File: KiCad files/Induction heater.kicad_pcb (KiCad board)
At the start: 2 copper layers, 100 x 100 mm, 31 parts, among them J1 PWR_IN, Q1 NMOS, Q2 NMOS, Q3 2N7000, Q4 2N7000, Q5 2N7000

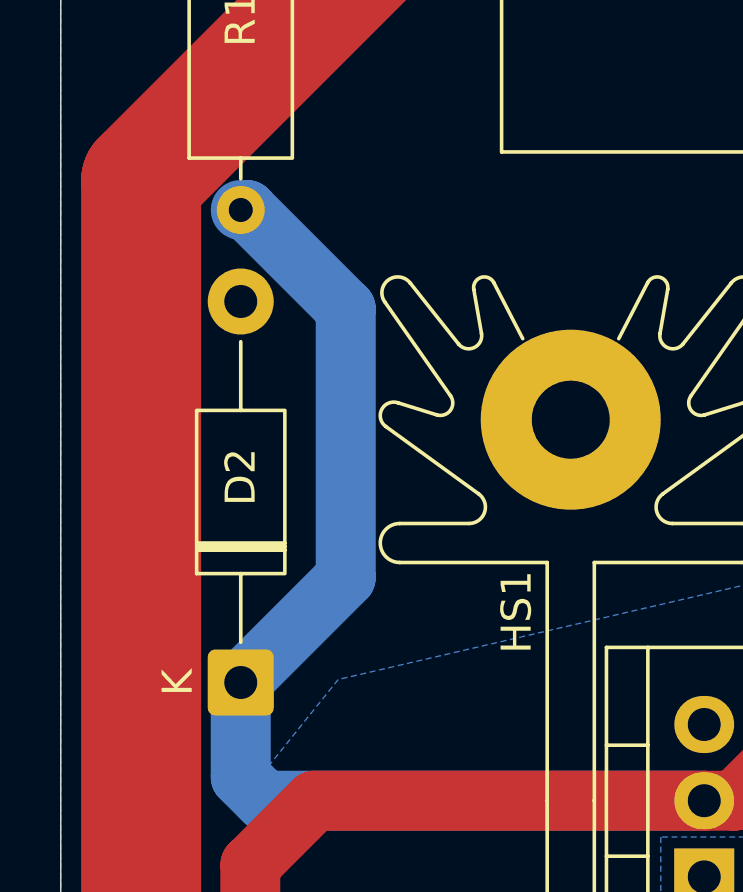
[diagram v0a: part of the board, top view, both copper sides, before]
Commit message: Update
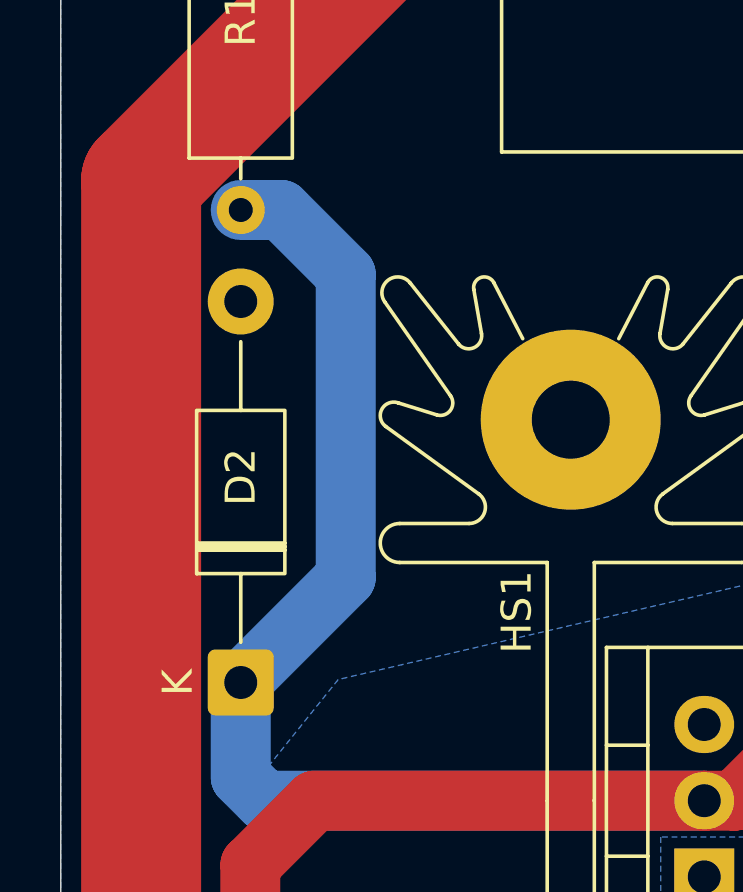
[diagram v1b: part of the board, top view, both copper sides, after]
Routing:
- net G2: track 148.5 -> 191.5 mm
- net G1: track 111.4 -> 150.4 mm
- net Net-(D3-K): track 68.3 -> 95.8 mm
- net Net-(D1-K): track 65.9 -> 78.0 mm
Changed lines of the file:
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@@
+	)
+	(segment
+		(start 104.22875 76.07625)
+		(end 110.555 69.75)
+		(width 3)
+		(layers "B.Cu" "B.Mask")
+		(solder_mask_margin 0)
+		(net 1)
 	)
 	(segment
@@
 	)
 	(segment
+		(start 101 76)
+		(end 104.1525 76)
+		(width 3)
+		(layers "B.Cu" "B.Mask")
+		(solder_mask_margin 0)
+		(net 1)
+	)
+	(segment
 		(start 108.25 118.35)
 		(end 107.35 119.25)
@@
 	)
 	(segment
+		(start 64.291315 76.07625)
+		(end 57.965065 69.75)
+		(width 3)
+		(layers "B.Cu" "B.Mask")
+		(solder_mask_margin 0)
+		(net 2)
+	)
+	(segment
+		(start 69.382121 76)
+		(end 64.577121 76)
+		(width 3)
+		(layers "B.Cu" "B.Mask")
+		(solder_mask_margin 0)
+		(net 2)
+	)
+	(segment
 		(start 58.0975 69.75)
 		(end 57.945 69.75)
@@
 	)
 	(segment
+		(start 69.172565 76)
+		(end 64.367565 76)
+		(width 3)
+		(layers "B.Cu" "B.Mask")
+		(solder_mask_margin 0)
+		(net 2)
+	)
+	(segment
+		(start 64.500871 76.07625)
+		(end 58.174621 69.75)
+		(width 3)
+		(layers "B.Cu" "B.Mask")
+		(solder_mask_margin 0)
+		(net 2)
+	)
+	(segment
 		(start 58.12 133.5)
 		(end 58.14 133.48)
@@
 	)
 	(segment
-		(start 44.25 94.85)
-		(end 44.25 85.895894)
-		(width 2)
-		(layer "B.Cu")
+		(start 42.1 82.6)
+		(end 40.75 82.6)
+		(width 2)
+		(layer "B.Cu")
+		(net 6)
+	)
+	(segment
+		(start 40.759429 101.5)
+		(end 40.759429 98.35)
+		(width 2)
+		(layers "B.Cu" "B.Mask")
+		(net 6)
+	)
+	(segment
+		(start 41.549429 102.29)
+		(end 40.759429 101.5)
+		(width 2)
+		(layers "B.Cu" "B.Mask")
 		(net 6)
 	)
@@
 	)
 	(segment
-		(start 44.25 94.85)
-		(end 40.75 98.35)
-		(width 2)
-		(layer "B.Cu")
-		(net 6)
-	)
-	(segment
-		(start 44.25 85.895894)
-		(end 40.954106 82.6)
-		(width 2)
-		(layer "B.Cu")
-		(net 6)
-	)
-	(segment
-		(start 40.954106 82.6)
-		(end 40.75 82.6)
-		(width 2)
-		(layer "B.Cu")
+		(start 40.75 98.35)
+		(end 44.25 94.85)
+		(width 2)
+		(layer "B.Cu")
+		(net 6)
+	)
+	(segment
+		(start 40.75 98.380338)
+		(end 44.25 94.880338)
+		(width 2)
+		(layers "B.Cu" "B.Mask")
 		(net 6)
 	)
@@
 	)
 	(segment
+		(start 44.25 84.780338)
+		(end 42.1 82.630338)
+		(width 2)
+		(layers "B.Cu" "B.Mask")
+		(net 6)
+	)
+	(segment
+		(start 56.209429 102.29)
+		(end 41.549429 102.29)
+		(width 2)
+		(layers "B.Cu" "B.Mask")
+		(net 6)
+	)
+	(segment
+		(start 44.25 84.75)
+		(end 42.1 82.6)
+		(width 2)
+		(layer "B.Cu")
+		(net 6)
+	)
+	(segment
+		(start 42.1 82.630338)
+		(end 40.75 82.630338)
+		(width 2)
+		(layers "B.Cu" "B.Mask")
+		(net 6)
+	)
+	(segment
+		(start 44.25 94.880338)
+		(end 44.25 84.780338)
+		(width 2)
+		(layers "B.Cu" "B.Mask")
+		(net 6)
+	)
+	(segment
+		(start 44.25 94.85)
+		(end 44.25 84.75)
+		(width 2)
+		(layer "B.Cu")
+		(net 6)
+	)
+	(segment
 		(start 41.54 102.29)
 		(end 40.75 101.5)
@@
 	)
 	(segment
+		(start 132.138708 84.696894)
+		(end 132.810688 85.368874)
+		(width 2)
+		(layers "B.Cu" "B.Mask")
+		(net 7)
+	)
+	(segment
 		(start 108.25 105.5)
 		(end 111.54 102.21)
@@
 	)
 	(segment
+		(start 132.810688 95.35)
+		(end 129.810688 98.35)
+		(width 2)
+		(layers "B.Cu" "B.Mask")
+		(net 7)
+	)
+	(segment
+		(start 111.522515 102.21)
+		(end 114.732515 102.21)
+		(width 2)
+		(layers "B.Cu" "B.Mask")
+		(net 7)
+	)
+	(segment
+		(start 132.111688 84.696894)
+		(end 132.138708 84.696894)
+		(width 2)
+		(layers "B.Cu" "B.Mask")
+		(net 7)
+	)
+	(segment
+		(start 108.232515 105.5)
+		(end 111.522515 102.21)
+		(width 2)
+		(layers "B.Cu" "B.Mask")
+		(net 7)
+	)
+	(segment
 		(start 132.051 84.696894)
 		(end 132.07802 84.696894)
@@
 	)
 	(segment
+		(start 125.865336 102.21)
+		(end 129.725336 98.35)
+		(width 2)
+		(layers "B.Cu" "B.Mask")
+		(net 7)
+	)
+	(segment
+		(start 130.014794 82.6)
+		(end 132.111688 84.696894)
+		(width 2)
+		(layers "B.Cu" "B.Mask")
+		(net 7)
+	)
+	(segment
+		(start 108.232515 105.65)
+		(end 108.232515 105.5)
+		(width 2)
+		(layers "B.Cu" "B.Mask")
+		(net 7)
+	)
+	(segment
+		(start 129.810688 82.6)
+		(end 130.014794 82.6)
+		(width 2)
+		(layers "B.Cu" "B.Mask")
+		(net 7)
+	)
+	(segment
 		(start 132.07802 84.696894)
 		(end 132.75 85.368874)
@@
 	)
 	(segment
+		(start 114.725336 102.21)
+		(end 125.865336 102.21)
+		(width 2)
+		(layers "B.Cu" "B.Mask")
+		(net 7)
+	)
+	(segment
 		(start 129.954106 82.6)
 		(end 132.051 84.696894)
@@
 		(net 7)
 	)
+	(segment
+		(start 132.810688 85.368874)
+		(end 132.810688 95.35)
+		(width 2)
+		(layers "B.Cu" "B.Mask")
+		(net 7)
+	)
